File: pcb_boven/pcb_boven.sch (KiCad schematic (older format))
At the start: 28 parts

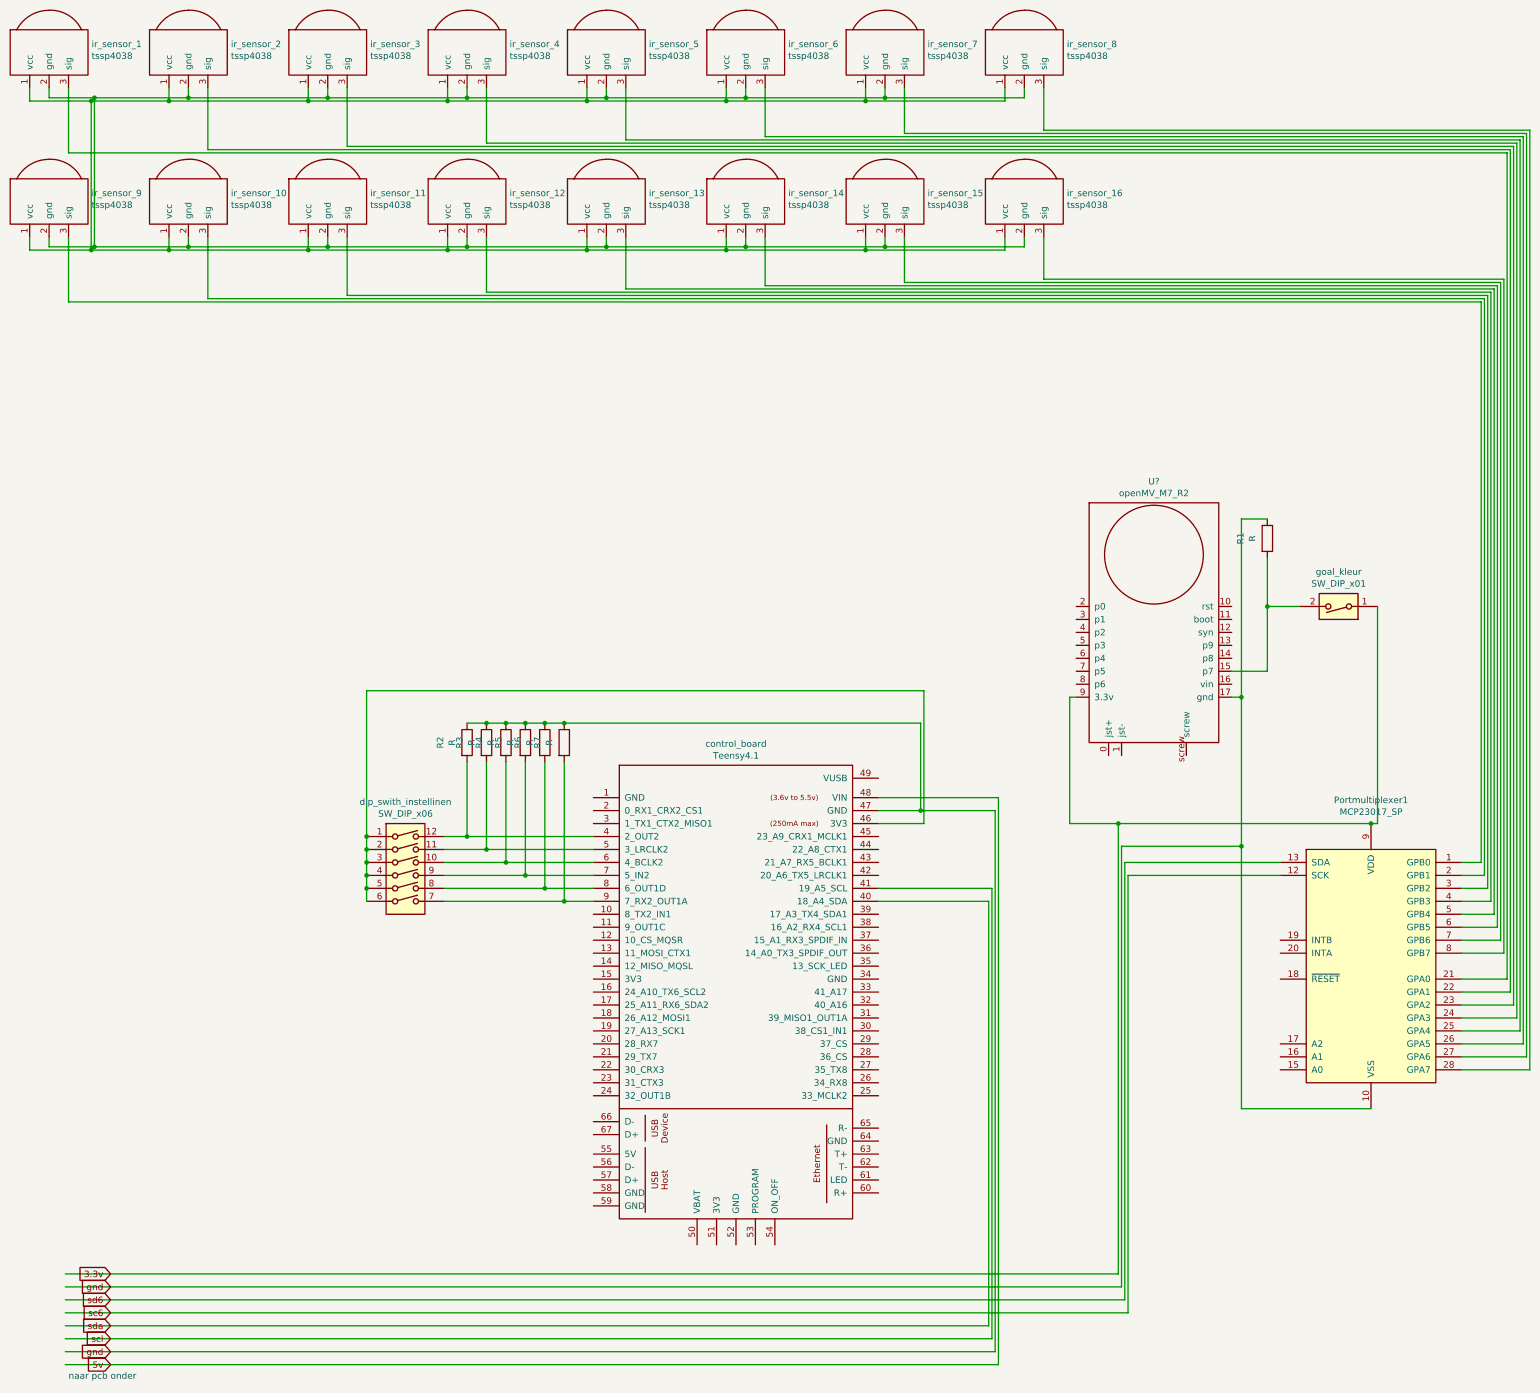
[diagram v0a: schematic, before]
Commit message: pcb onder gemaakt
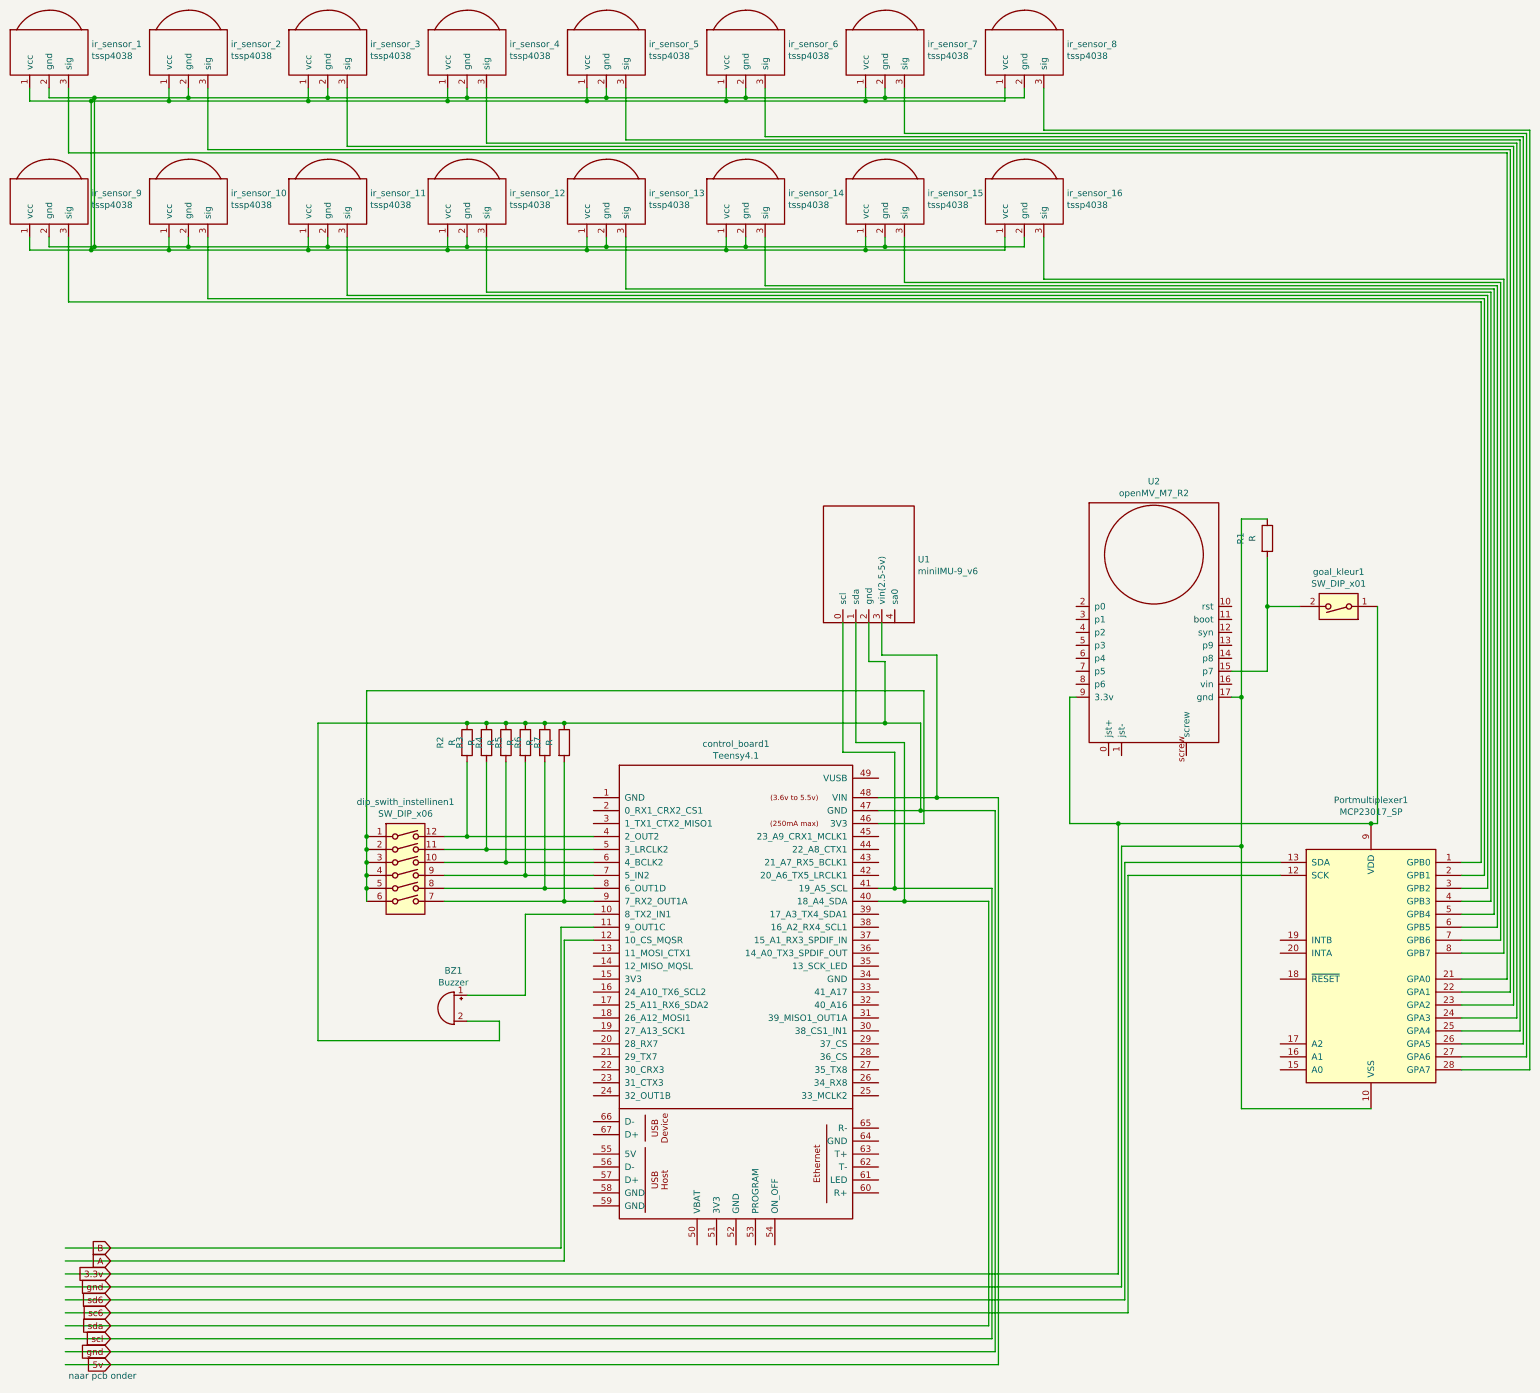
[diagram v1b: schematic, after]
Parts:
- added BZ1: Buzzer, symbol Device:Buzzer
- added U1: miniIMU-9_v6, custom:miniIMU-9_v6, symbol miniimu-9_v6:miniIMU-9_v6
- gave numbers to parts that had none: 1
- renumbered control_board to control_board1, dip_swith_instellinen to dip_swith_instellinen1, goal_kleur to goal_kleur1
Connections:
- net labels added: A, B
- wire segments 204 -> 234
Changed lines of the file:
@@
 $EndDescr
 $Comp
-L openmv_m7_r2:openMV_M7_R2 U?
+L openmv_m7_r2:openMV_M7_R2 U2
 U 1 1 66360711
 P 9350 5325
-F 0 "U?" H 9350 6490 50  0000 C CNN
+F 0 "U2" H 9350 6490 50  0000 C CNN
 F 1 "openMV_M7_R2" H 9350 6399 50  0000 C CNN
 F 2 "custom:openmv_m7_r2" H 9350 6675 50  0001 C CNN
@@
 $EndComp
 $Comp
-L teensy:Teensy4.1 control_board
+L teensy:Teensy4.1 control_board1
 U 1 1 66362D60
 P 6125 8750
-F 0 "control_board" H 6125 11315 50  0000 C CNN
+F 0 "control_board1" H 6125 11315 50  0000 C CNN
 F 1 "Teensy4.1" H 6125 11224 50  0000 C CNN
 F 2 "" H 5725 9150 50  0001 C CNN
@@
 $EndComp
 $Comp
-L Switch:SW_DIP_x06 dip_swith_instellinen
+L Switch:SW_DIP_x06 dip_swith_instellinen1
 U 1 1 66364D70
 P 3575 7200
-F 0 "dip_swith_instellinen" H 3575 7767 50  0000 C CNN
+F 0 "dip_swith_instellinen1" H 3575 7767 50  0000 C CNN
 F 1 "SW_DIP_x06" H 3575 7676 50  0000 C CNN
 F 2 "" H 3575 7200 50  0001 C CNN
@@
 $EndComp
 $Comp
-L Switch:SW_DIP_x01 goal_kleur
+L Switch:SW_DIP_x01 goal_kleur1
 U 1 1 66365885
 P 10775 5125
-F 0 "goal_kleur" H 10775 4858 50  0000 C CNN
+F 0 "goal_kleur1" H 10775 4858 50  0000 C CNN
 F 1 "SW_DIP_x01" H 10775 4949 50  0000 C CNN
 F 2 "" H 10775 5125 50  0001 C CNN
@@
 $EndComp
 Wire Wire Line
-	7225 7300 8100 7300
+	7225 7300 7350 7300
 Wire Wire Line
 	8100 7300 8100 10775
@@
 scl
 Wire Wire Line
-	7225 7400 8075 7400
+	7225 7400 7425 7400
 Wire Wire Line
 	8075 7400 8075 10675
@@
 gnd
 Wire Wire Line
-	7225 6600 8150 6600
+	7225 6600 7675 6600
 Wire Wire Line
 	8150 6600 8150 10975
@@
 Connection ~ 4200 6025
 Wire Wire Line
-	4800 6025 7550 6025
+	4800 6025 7275 6025
 Wire Wire Line
 	7550 6025 7550 6700
@@
 	10025 4450 10025 5825
 Connection ~ 10025 5825
+$Comp
+L Device:Buzzer BZ1
+U 1 1 663737AA
+P 3950 8225
+F 0 "BZ1" H 3955 8515 50  0000 C CNN
+F 1 "Buzzer" H 3955 8424 50  0000 C CNN
+F 2 "" V 3925 8325 50  0001 C CNN
+F 3 "~" V 3925 8325 50  0001 C CNN
+	1    3950 8225
+	-1   0    0    -1
+$EndComp
+Wire Wire Line
+	4050 8125 4500 8125
+Wire Wire Line
+	4500 8125 4500 7500
+Wire Wire Line
+	4500 7500 5025 7500
+Wire Wire Line
+	2900 6025 4050 6025
+Wire Wire Line
+	4050 8325 4300 8325
+Connection ~ 4050 6025
+Wire Wire Line
+	2900 8475 4300 8475
+Wire Wire Line
+	4300 8475 4300 8325
+Wire Wire Line
+	2900 6025 2900 8475
+$Comp
+L miniimu-9_v6:miniIMU-9_v6 U1
+U 1 1 663B967A
+P 7050 4650
+F 0 "U1" H 7528 4538 50  0000 L CNN
+F 1 "miniIMU-9_v6" H 7528 4447 50  0000 L CNN
+F 2 "custom:miniIMU-9_v6" H 7050 5100 50  0001 C CNN
+F 3 "" H 7050 5100 50  0001 C CNN
+	1    7050 4650
+	1    0    0    -1
+$EndComp
+Wire Wire Line
+	7150 5250 7150 5550
+Wire Wire Line
+	7150 5550 7275 5550
+Wire Wire Line
+	7275 5550 7275 6025
+Connection ~ 7275 6025
+Wire Wire Line
+	7275 6025 7550 6025
+Wire Wire Line
+	7675 6600 7675 5500
+Wire Wire Line
+	7675 5500 7250 5500
+Wire Wire Line
+	7250 5500 7250 5250
+Connection ~ 7675 6600
+Wire Wire Line
+	7675 6600 8150 6600
+Wire Wire Line
+	7050 5250 7050 6175
+Wire Wire Line
+	7050 6175 7425 6175
+Wire Wire Line
+	7425 6175 7425 7400
+Connection ~ 7425 7400
+Wire Wire Line
+	7425 7400 8075 7400
+Wire Wire Line
+	7350 7300 7350 6250
+Wire Wire Line
+	7350 6250 6950 6250
+Wire Wire Line
+	6950 6250 6950 5250
+Connection ~ 7350 7300
+Wire Wire Line
+	7350 7300 8100 7300
+Text GLabel 1300 10175 0    50   Input ~ 0
+A
+Text GLabel 1300 10075 0    50   Input ~ 0
+B
+Wire Wire Line
+	4800 7700 5025 7700
+Wire Wire Line
+	950  10175 4800 10175
+Wire Wire Line
+	4800 10175 4800 7700
+Wire Wire Line
+	5025 7600 4775 7600
+Wire Wire Line
+	4775 7600 4775 10075
+Wire Wire Line
+	4775 10075 950  10075
 $EndSCHEMATC

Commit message: pcb onder gemaakt
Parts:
- BZ1: footprint (none) -> custom:buzer
- control_board1: footprint (none) -> custom:teensy4.1
- dip_swith_instellinen1: footprint (none) -> custom:dipswitch6
- goal_kleur1: footprint (none) -> custom:dipswitch1
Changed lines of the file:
@@
 F 0 "control_board1" H 6125 11315 50  0000 C CNN
 F 1 "Teensy4.1" H 6125 11224 50  0000 C CNN
-F 2 "" H 5725 9150 50  0001 C CNN
+F 2 "custom:teensy4.1" H 5725 9150 50  0001 C CNN
 F 3 "" H 5725 9150 50  0001 C CNN
 	1    6125 8750
@@
 F 0 "dip_swith_instellinen1" H 3575 7767 50  0000 C CNN
 F 1 "SW_DIP_x06" H 3575 7676 50  0000 C CNN
-F 2 "" H 3575 7200 50  0001 C CNN
+F 2 "custom:dipswitch6" H 3575 7200 50  0001 C CNN
 F 3 "~" H 3575 7200 50  0001 C CNN
 	1    3575 7200
@@
 F 0 "goal_kleur1" H 10775 4858 50  0000 C CNN
 F 1 "SW_DIP_x01" H 10775 4949 50  0000 C CNN
-F 2 "" H 10775 5125 50  0001 C CNN
+F 2 "custom:dipswitch1" H 10775 5125 50  0001 C CNN
 F 3 "~" H 10775 5125 50  0001 C CNN
 	1    10775 5125
@@
 F 0 "BZ1" H 3955 8515 50  0000 C CNN
 F 1 "Buzzer" H 3955 8424 50  0000 C CNN
-F 2 "" V 3925 8325 50  0001 C CNN
+F 2 "custom:buzer" V 3925 8325 50  0001 C CNN
 F 3 "~" V 3925 8325 50  0001 C CNN
 	1    3950 8225
